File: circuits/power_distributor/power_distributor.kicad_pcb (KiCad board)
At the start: 2 copper layers, 73.7 x 39.4 mm, 12 parts, among them P1 CONN_01X02, P2 CONN_01X02, P3 CONN_01X02, P4 CONN_01X02, P5 CONN_01X02, P6 CONN_01X01, P7 CONN_01X01, P8 CONN_01X01, P9 CONN_01X01, U1 LD1117S33TR

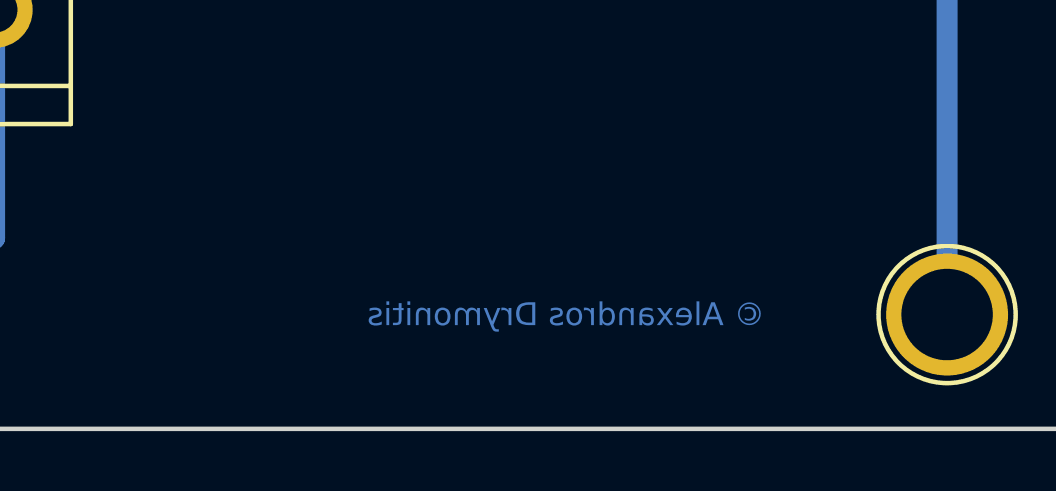
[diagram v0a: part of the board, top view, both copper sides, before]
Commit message: Update circuits
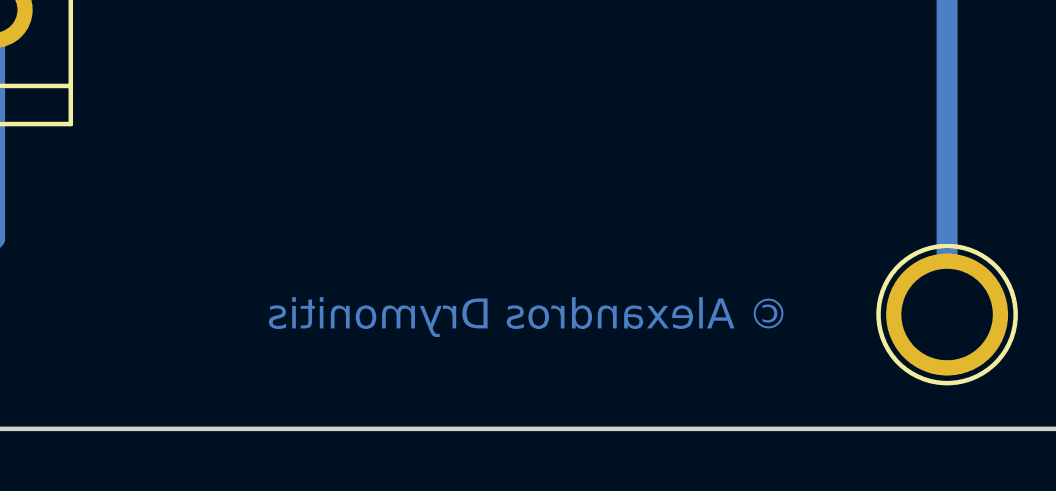
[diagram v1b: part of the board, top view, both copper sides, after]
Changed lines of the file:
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@@
-(kicad_pcb (version 4) (host pcbnew 4.0.2+dfsg1-2~bpo8+1-stable)
+(kicad_pcb (version 4) (host pcbnew 4.0.6+dfsg1-1)
   (general
     (links 18)
     (no_connects 0)
-    (area 114.224999 85.014999 188.035001 124.535001)
+    (area 113.076667 84.115 189.183334 124.535001)
     (thickness 1.6)
     (drawings 5)
@@
   (title_block
     (title "Modular Synthesizer Power Distributor")
-    (date 2017-07-12)
+    (date 2017-11-01)
+    (rev 1)
     (company "Alexandros Drymonitis")
   )
@@
     (visible_elements FFFFFF7F)
     (pcbplotparams
-      (layerselection 0x00030_80000001)
+      (layerselection 0x010f0_80000001)
       (usegerberextensions false)
       (excludeedgelayer true)
@@
       (outputformat 1)
       (mirror false)
-      (drillshape 1)
+      (drillshape 0)
       (scaleselection 1)
-      (outputdirectory ""))
+      (outputdirectory ../../../../Documents/kicad/3dPd/power_distributor/svg_files/))
   )
   (net 0 "")
@@
       (net 2 GND))
   )
-  (gr_text "© Alexandros Drymonitis" (at 171.45 120.65) (layer B.Cu)
-    (effects (font (size 0.762 0.762) (thickness 0.1905)) (justify mirror))
+  (gr_text "© Alexandros Drymonitis" (at 170.18 120.65) (layer B.Cu)
+    (effects (font (size 1 1) (thickness 0.1905)) (justify mirror))
   )
   (gr_line (start 187.96 124.46) (end 187.96 85.09) (angle 90) (layer Edge.Cuts) (width 0.15))
@@
     (polygon
       (pts
-        (xy 187.96 124.46) (xy 114.3 124.46) (xy 114.3 85.09) (xy 187.96 85.09) (xy 187.96 124.46)
+        (xy 187.96 124.46) (xy 114.3 124.46) (xy 114.3 85.09) (xy 187.96 85.09)
       )
     )
